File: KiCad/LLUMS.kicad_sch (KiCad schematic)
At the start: 38 parts, among them J7 Conn_01x10_Pin, Q1 AO3400A, Q2 AO3400A, Q3 AO3400A, Q4 AO3400A, Q5 AO3400A, Q6 AO3400A, Q7 AO3400A, Q8 AO3400A, U9 RPR-0521RS

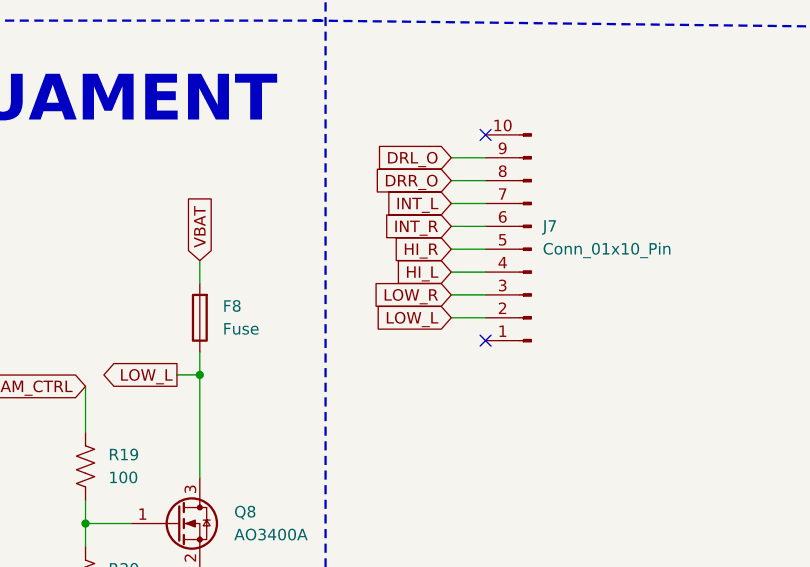
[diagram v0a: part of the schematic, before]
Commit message: Placa
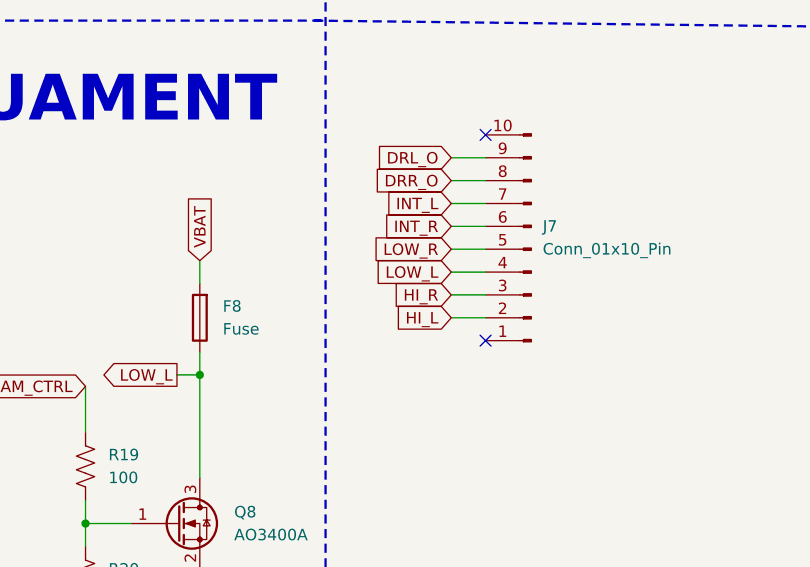
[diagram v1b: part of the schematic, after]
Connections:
- net HI_L: now also J7.2 (Pin_2); no longer J7.4 (Pin_4)
- net HI_R: now also J7.3 (Pin_3); no longer J7.5 (Pin_5)
- net LOW_L: now also J7.4 (Pin_4); no longer J7.2 (Pin_2)
- net LOW_R: now also J7.5 (Pin_5); no longer J7.3 (Pin_3)
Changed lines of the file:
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@@
-		)
-	)
-	(global_label "LOW_L"
-		(shape input)
-		(at 190.5 135.89 180)
-		(fields_autoplaced yes)
-		(effects
-			(font
-				(size 1.27 1.27)
-			)
-			(justify right)
-		)
-		(property "Intersheetrefs" "${INTERSHEET_REFS}"
-			(at 181.7091 135.89 0)
-			(effects
-				(font
-					(size 1.27 1.27)
-				)
-				(justify right)
-				(hide yes)
-			)
 		)
 	)
@@
 		)
 	)
+	(global_label "LOW_R"
+		(shape input)
+		(at 190.5 128.27 180)
+		(fields_autoplaced yes)
+		(effects
+			(font
+				(size 1.27 1.27)
+			)
+			(justify right)
+		)
+		(property "Intersheetrefs" "${INTERSHEET_REFS}"
+			(at 181.4672 128.27 0)
+			(effects
+				(font
+					(size 1.27 1.27)
+				)
+				(justify right)
+				(hide yes)
+			)
+		)
+	)
 	(global_label "VCC"
 		(shape input)
@@
 				)
 				(justify left)
-				(hide yes)
-			)
-		)
-	)
-	(global_label "HI_L"
-		(shape input)
-		(at 190.5 130.81 180)
-		(fields_autoplaced yes)
-		(effects
-			(font
-				(size 1.27 1.27)
-			)
-			(justify right)
-		)
-		(property "Intersheetrefs" "${INTERSHEET_REFS}"
-			(at 183.5838 130.81 0)
-			(effects
-				(font
-					(size 1.27 1.27)
-				)
-				(justify right)
 				(hide yes)
 			)
@@
 		)
 	)
-	(global_label "LOW_R"
-		(shape input)
-		(at 190.5 133.35 180)
-		(fields_autoplaced yes)
-		(effects
-			(font
-				(size 1.27 1.27)
-			)
-			(justify right)
-		)
-		(property "Intersheetrefs" "${INTERSHEET_REFS}"
-			(at 181.4672 133.35 0)
-			(effects
-				(font
-					(size 1.27 1.27)
-				)
-				(justify right)
-				(hide yes)
-			)
-		)
-	)
 	(global_label "HI_BEAM_CTRL"
 		(shape input)
@@
 		)
 	)
+	(global_label "HI_L"
+		(shape input)
+		(at 190.5 135.89 180)
+		(fields_autoplaced yes)
+		(effects
+			(font
+				(size 1.27 1.27)
+			)
+			(justify right)
+		)
+		(property "Intersheetrefs" "${INTERSHEET_REFS}"
+			(at 183.5838 135.89 0)
+			(effects
+				(font
+					(size 1.27 1.27)
+				)
+				(justify right)
+				(hide yes)
+			)
+		)
+	)
 	(global_label "DRL_O"
 		(shape output)
@@
 		)
 	)
+	(global_label "LOW_L"
+		(shape input)
+		(at 190.5 130.81 180)
+		(fields_autoplaced yes)
+		(effects
+			(font
+				(size 1.27 1.27)
+			)
+			(justify right)
+		)
+		(property "Intersheetrefs" "${INTERSHEET_REFS}"
+			(at 181.7091 130.81 0)
+			(effects
+				(font
+					(size 1.27 1.27)
+				)
+				(justify right)
+				(hide yes)
+			)
+		)
+	)
+	(global_label "SCL"
+		(shape input)
+		(at 212.09 67.31 180)
+		(fields_autoplaced yes)
+		(effects
+			(font
+				(size 1.27 1.27)
+			)
+			(justify right)
+		)
+		(property "Intersheetrefs" "${INTERSHEET_REFS}"
+			(at 205.5972 67.31 0)
+			(effects
+				(font
+					(size 1.27 1.27)
+				)
+				(justify right)
+				(hide yes)
+			)
+		)
+	)
 	(global_label "HI_R"
 		(shape input)
-		(at 190.5 128.27 180)
-		(fields_autoplaced yes)
-		(effects
-			(font
-				(size 1.27 1.27)
-			)
-			(justify right)
-		)
-		(property "Intersheetrefs" "${INTERSHEET_REFS}"
-			(at 183.3419 128.27 0)
-			(effects
-				(font
-					(size 1.27 1.27)
-				)
-				(justify right)
-				(hide yes)
-			)
-		)
-	)
-	(global_label "SCL"
-		(shape input)
-		(at 212.09 67.31 180)
-		(fields_autoplaced yes)
-		(effects
-			(font
-				(size 1.27 1.27)
-			)
-			(justify right)
-		)
-		(property "Intersheetrefs" "${INTERSHEET_REFS}"
-			(at 205.5972 67.31 0)
-			(effects
-				(font
+		(at 190.5 133.35 180)
+		(fields_autoplaced yes)
+		(effects
+			(font
+				(size 1.27 1.27)
+			)
+			(justify right)
+		)
+		(property "Intersheetrefs" "${INTERSHEET_REFS}"
+			(at 183.3419 133.35 0)
+			(effects
+				(font

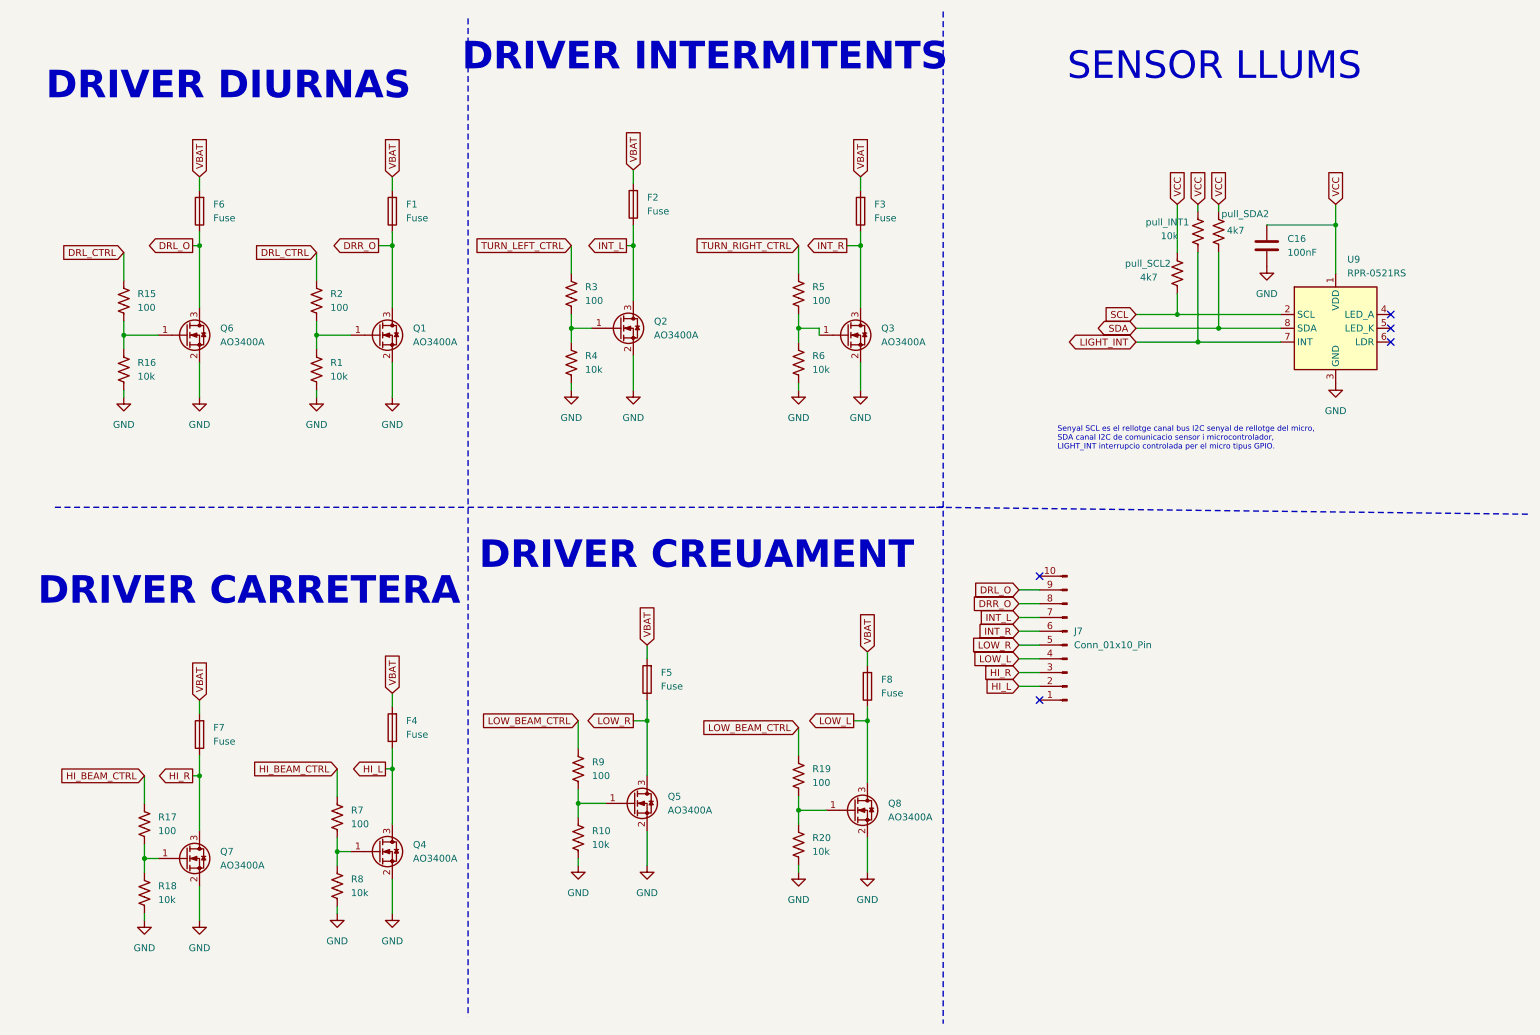
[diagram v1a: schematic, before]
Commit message: a
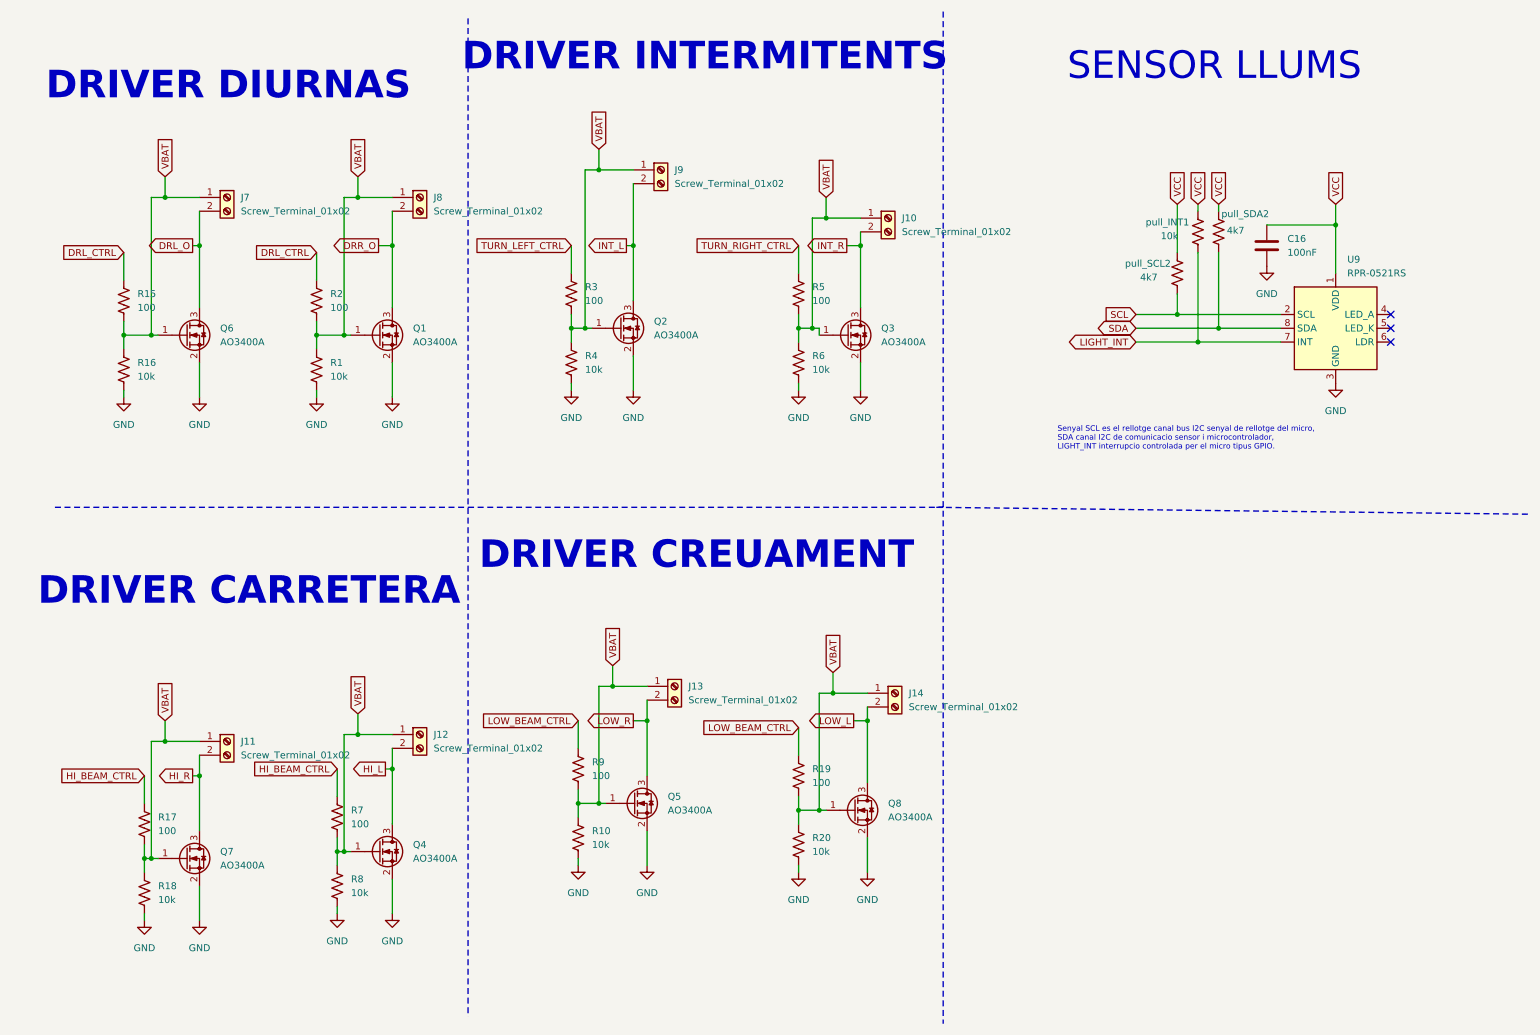
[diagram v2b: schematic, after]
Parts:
- removed F1, F2, F3, F4, F5, F6, F7, F8: Fuse, Fuse:Fuse_0805_2012Metric, symbol Device:Fuse
- removed J7: Conn_01x10_Pin, Connector_PinHeader_2.54mm:PinHeader_1x10_P2.54mm_Vertical, symbol Connector:Conn_01x10_Pin
- added J10, J11, J12, J13, J14, J7, J8, J9: Screw_Terminal_01x02, TerminalBlock_Phoenix:TerminalBlock_Phoenix_MKDS-1,5-2-5.08_1x02_P5.08mm_Horizontal, symbol Connector:Screw_Terminal_01x02
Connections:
- net DRL_O: now also J7.2 (Pin_2)
- net DRR_O: now also J8.2 (Pin_2)
- net HI_L: now also J12.2 (Pin_2)
- net HI_R: now also J11.2 (Pin_2)
- net INT_L: now also J9.2 (Pin_2)
- net INT_R: now also J10.2 (Pin_2)
- net LOW_L: now also J14.2 (Pin_2)
- net LOW_R: now also J13.2 (Pin_2)
- net VBAT: now also Q1.1 (G), Q2.1 (G), Q3.1 (G), Q4.1 (G), Q5.1 (G), Q6.1 (G), Q7.1 (G), Q8.1 (G), R1.1, R10.1, R15.2, R16.1, R17.2, R18.1, R19.2, R2.2, R20.1, R3.2, R4.1, R5.2, R6.1, R7.2, R8.1, R9.2, J10.1 (Pin_1), J11.1 (Pin_1), J12.1 (Pin_1), J13.1 (Pin_1), J14.1 (Pin_1), J7.1 (Pin_1), J8.1 (Pin_1), J9.1 (Pin_1)
- no-connect marks 5 -> 3
